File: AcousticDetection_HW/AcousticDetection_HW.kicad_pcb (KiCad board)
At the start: 2 copper layers, 208 x 44 mm, 41 parts, among them J1 USB_C_Receptacle_USB2.0, J10 PWR_R, J11 DATA_R, J12 DATA_R, J3 UART, J4 JTAG, J5 PWR_L, J6 PWR_L, J7 DATA_L, J8 DATA_L, J9 PWR_R, SW1 EN, SW2 BOOT, U1 ESP32-WROOM-32, U2 LDL1117S33R_SOT223

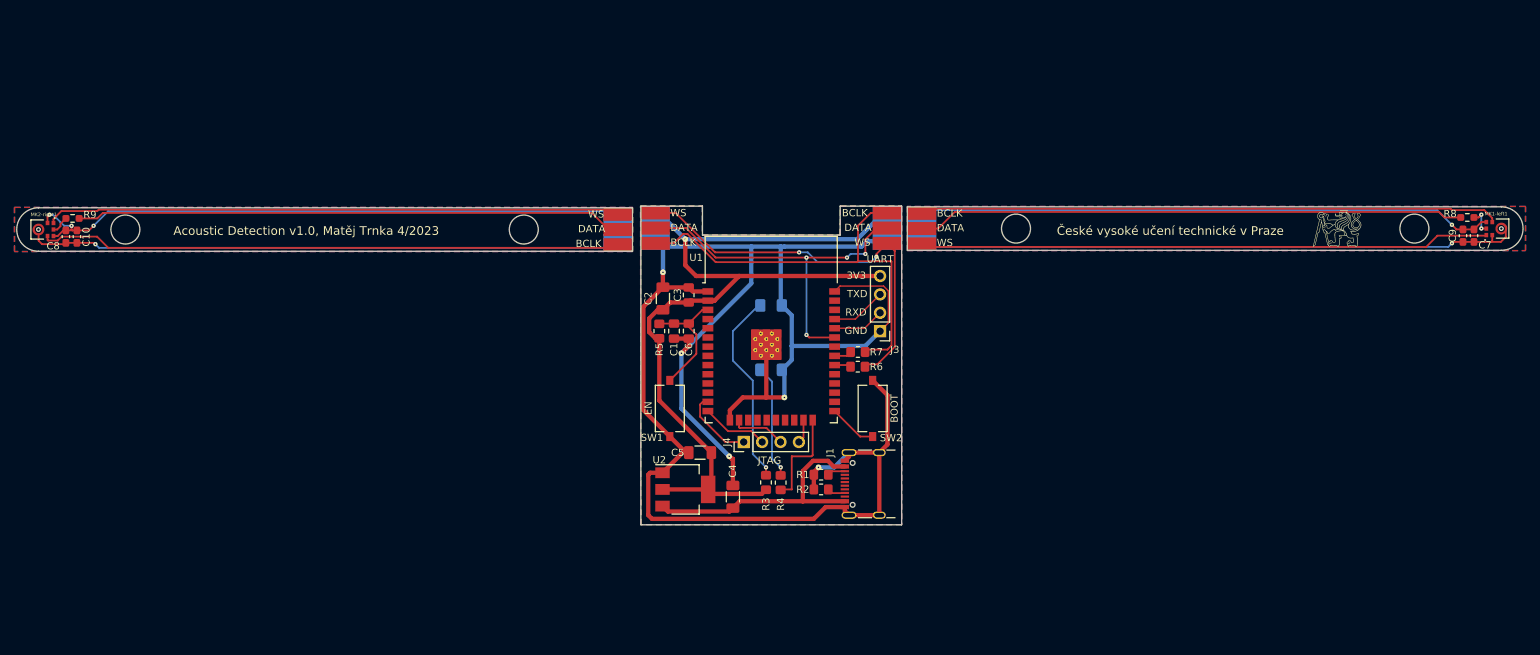
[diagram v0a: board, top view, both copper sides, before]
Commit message: parts labels reposition
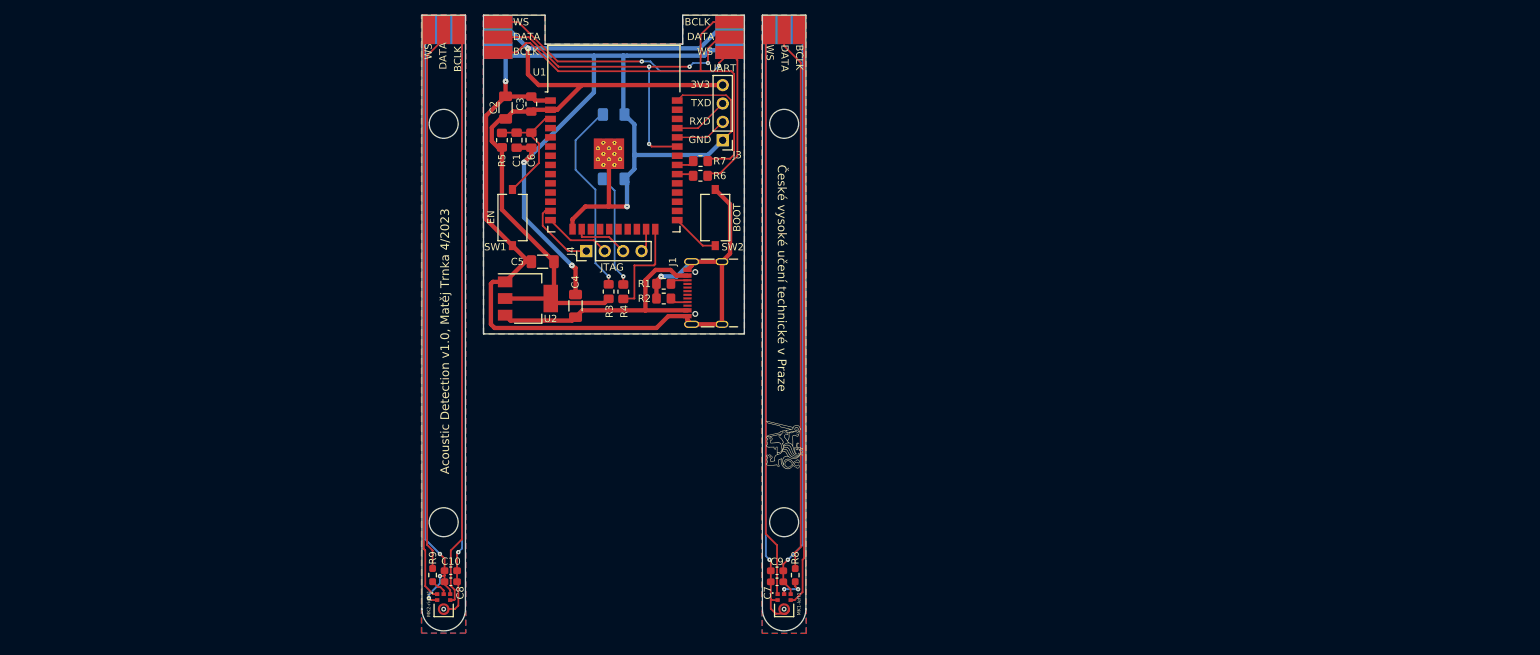
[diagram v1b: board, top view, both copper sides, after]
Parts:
- moved G*** 112.5 mm to (146.3, 135.6), turned to 90 degrees
- moved MK1-left1 112.1 mm to (146.3, 135.3), turned to 0 degrees
- moved C7 107.4 mm to (145.3, 131.6), turned to 0 degrees
- moved C9 105.4 mm to (145.3, 130.0), turned to 0 degrees
- moved R8 105.1 mm to (147.8, 130.7), turned to 90 degrees
- moved G*** 77.0 mm to (99.3, 135.6), turned to -90 degrees
- moved MK2-right1 76.7 mm to (99.3, 135.3), turned to 0 degrees
- moved C8 71.4 mm to (100.3, 131.6), turned to 180 degrees
- moved R9 70.0 mm to (97.8, 130.6), turned to 90 degrees
- moved C10 69.2 mm to (100.3, 130.0), turned to 180 degrees
- moved J10 36.6 mm to (99.3, 55.3), turned to -90 degrees
- moved J12 36.6 mm to (99.3, 55.3), turned to -90 degrees
- moved C1 34.2 mm to (109.4, 70.6)
- moved R1 34.2 mm to (129.7, 90.4)
- moved R2 34.2 mm to (129.7, 92.5)
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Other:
- board size 208 x 44 mm -> 53 x 85 mm

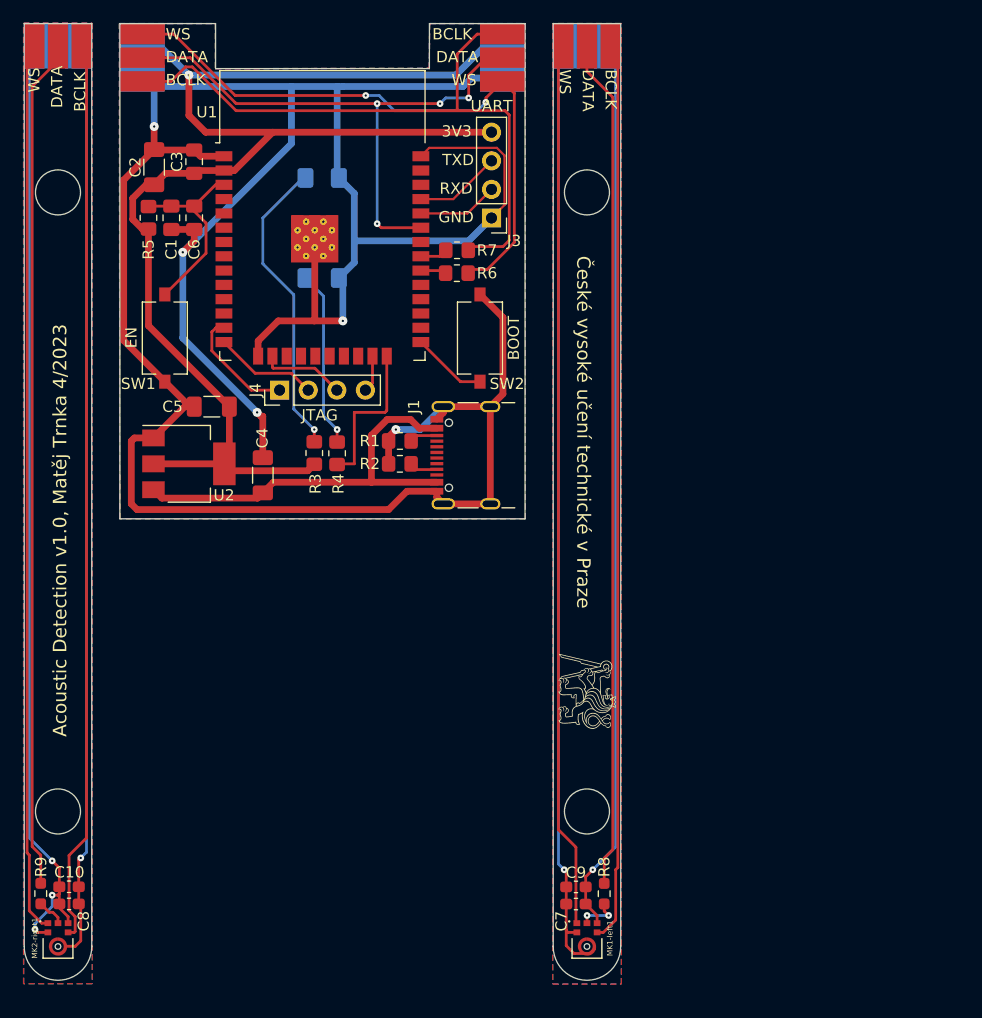
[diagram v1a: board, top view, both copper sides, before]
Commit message: pcb fabrication
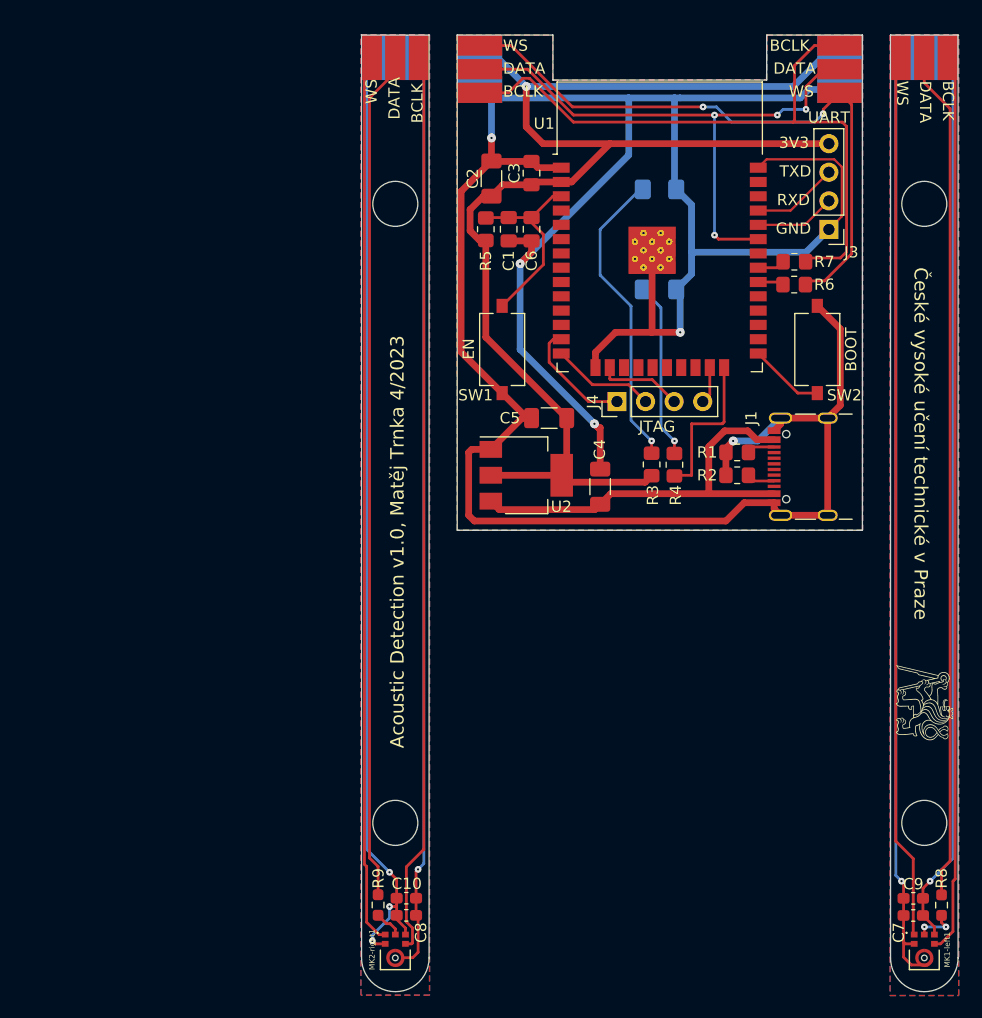
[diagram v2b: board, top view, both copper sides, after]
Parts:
- moved C1 30.0 mm to (139.3, 71.6)
- moved C2 30.0 mm to (137.8, 67.1)
- moved C5 30.0 mm to (142.9, 88.4)
- moved C6 30.0 mm to (141.4, 71.6)
- moved C7 30.0 mm to (175.3, 132.6)
- moved C9 30.0 mm to (175.3, 131.1)
- moved D1 30.0 mm to (152.7, 68.1)
- moved D2 30.0 mm to (152.7, 77.0)
- moved G*** 30.0 mm to (176.3, 136.7)
- moved G*** 30.0 mm to (144.7, 93.2)
- moved J1 30.0 mm to (166.6, 92.7)
- moved J11 30.0 mm to (136.8, 57.4)
- moved J3 30.0 mm to (167.8, 71.6)
- moved J5 30.0 mm to (168.8, 57.4)
- moved J6 30.0 mm to (176.3, 56.4)
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
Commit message: the resistor values of pcb leds were changed to 220R
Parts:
- R3, R4: value 1k -> 220R
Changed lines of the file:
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@@
         (effects (font (size 1 1) (thickness 0.15)))
     )
-    (fp_text value "1k" (at 0 1.65 90) (layer "F.Fab")
+    (fp_text value "220R" (at 0 1.65 90) (layer "F.Fab")
         (effects (font (size 1 1) (thickness 0.15)))
     )
@@
         (effects (font (size 1 1) (thickness 0.15)))
     )
-    (fp_text value "1k" (at 0 1.65 90) (layer "F.Fab")
-        (effects (font (size 1 1) (thickness 0.15)))
-    )
+    (fp_text value "220R" (at 0 1.65 90) (layer "F.Fab")
+        (effects (font (size 1 1) (thickness 0.15)))
+    )
